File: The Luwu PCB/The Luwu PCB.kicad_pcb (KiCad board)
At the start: 4 copper layers, 38.3 x 104.3 mm, 81 parts, among them IC1 TPS22953DSQR, IC2 ESP32-C3FH4, IC4 CD40109BPWR, IC5 SN74LV1T04DCKRG4, IC6 UCC27519DBVR, IC7 UCC27519DBVR, IC8 UCC27519DBVR, J1 2337019-1, J10 Neopixel Terminal out 3, J2 USB_C_Receptacle_USB2.0, J3 5V_IN, J4 Neopixel Terminal opt 1, J5 12V_IN, J6 V SEL LS, J7 Screw_Terminal_01x04, J8 Neopixel Terminal, J9 Neopixel Terminal opt 2, Q2 BUK7D25-40EX, Q3 BUK7D25-40EX, Q4 BUK7D25-40EX, SW1 PTS636 SP50, SW2 PTS636 SP50, U1 2.4GHZ_PCB_Antenna_AN043, U2 AP2112K-3.3, U3 USBLC6-2SC6, Y1 ECS-400-10-37B2-CKM-TR

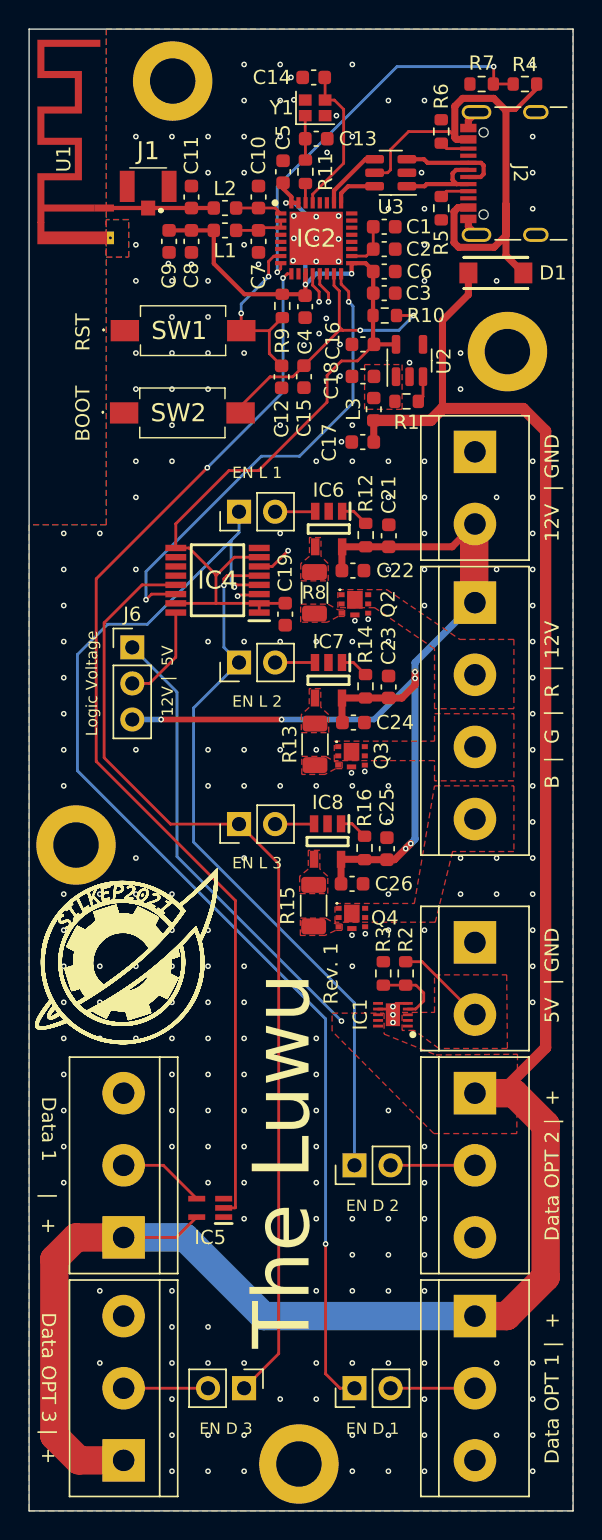
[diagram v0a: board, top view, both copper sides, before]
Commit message: updated size
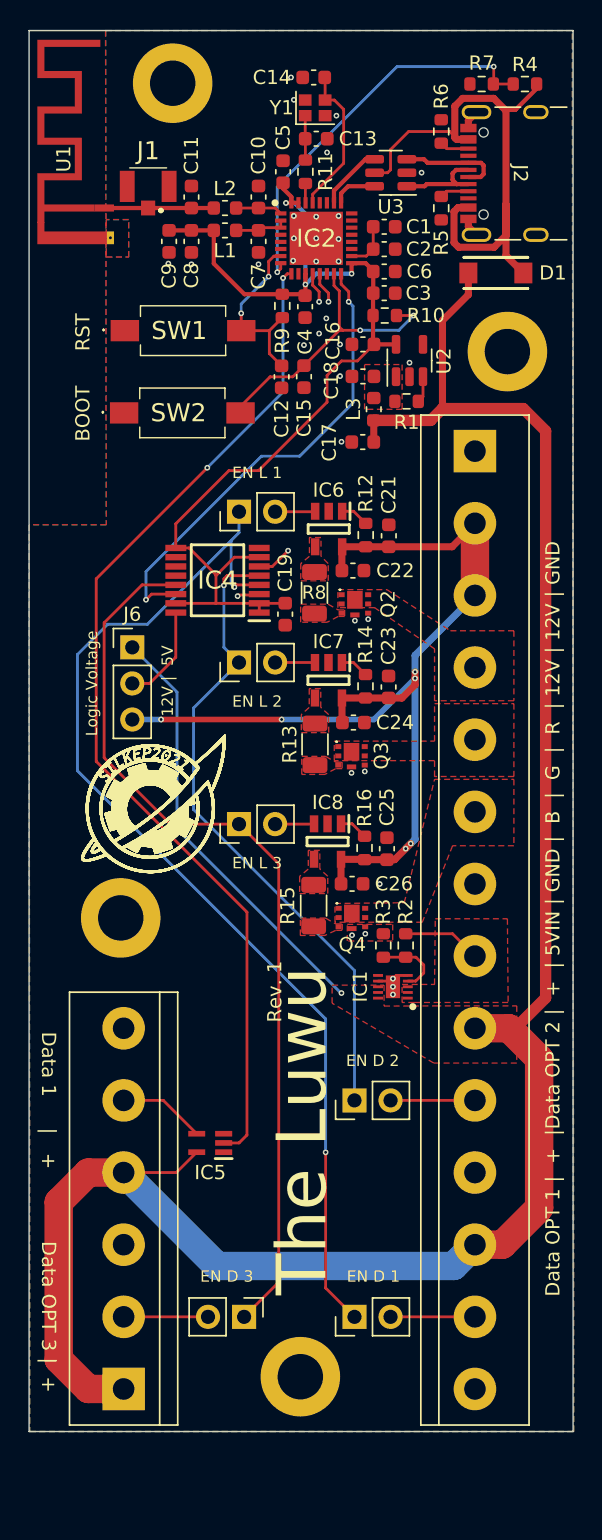
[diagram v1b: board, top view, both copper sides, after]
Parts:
- removed J10: Neopixel Terminal out 3, TerminalBlock:TerminalBlock_bornier-3_P5.08mm
- removed J3: 5V_IN, TerminalBlock:TerminalBlock_bornier-2_P5.08mm
- removed J5: 12V_IN, TerminalBlock:TerminalBlock_bornier-2_P5.08mm
- removed J7: Screw_Terminal_01x04, TerminalBlock:TerminalBlock_bornier-4_P5.08mm
- removed J8: Neopixel Terminal, TerminalBlock:TerminalBlock_bornier-3_P5.08mm
- removed J9: Neopixel Terminal opt 2, TerminalBlock:TerminalBlock_bornier-3_P5.08mm
- added J11: Screw_Terminal_01x14, Connector_custom:TerminalBlock_bornier-14_P5.08mm, F.Cu at (98.2, 111.3)
- J4: value Neopixel Terminal opt 1 -> Screw_Terminal_01x06; footprint TerminalBlock:TerminalBlock_bornier-3_P5.08mm -> TerminalBlock:TerminalBlock_bornier-6_P5.08mm
- moved J4 25.3 mm to (73.5, 146.9), turned to 90 degrees
- moved H3 6.15 mm to (85.9, 146.0)
- moved H1 6.02 mm to (73.3, 113.7)
- moved JP1 5.03 mm to (89.7, 141.8)
- moved JP3 5.03 mm to (81.9, 141.8)
- moved IC5 4.57 mm to (79.6, 129.5)
- moved JP2 4.57 mm to (89.7, 126.5)
- moved IC1 1.97 mm to (92.4, 118.5)
- moved R2 1.97 mm to (93.3, 115.6)
- moved R3 1.97 mm to (91.7, 115.6)
- moved H4 0.15 mm to (76.9, 54.9)
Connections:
- net /5V_IN_TERM renamed 5V_IN_TERM
- IC5 pad 4: /DATA 1 OUT -> DATA 1 OUT
- J4 pad 2: /DATA OPT1 OUT -> DATA OPT3 OUT
- JP1 pad 2: /DATA OPT1 OUT -> DATA OPT1 OUT
- JP2 pad 2: /DATA OPT2 OUT -> DATA OPT2 OUT
- JP3 pad 2: /DATA OPT3 OUT -> DATA OPT3 OUT
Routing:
- net +5V: track 186.1 -> 178.5 mm
- net DATA 1 OUT: track 0.00 -> 6.12 mm
- net /DATA 1 OUT: track 6.12 -> 0.00 mm
- net DATA OPT3 OUT: track 0.00 -> 5.94 mm
- net DATA OPT2 OUT: track 0.00 -> 5.94 mm
- net DATA OPT1 OUT: track 0.00 -> 5.94 mm
- net /DATA OPT3 OUT: track 5.94 -> 0.00 mm
- net /DATA OPT2 OUT: track 5.94 -> 0.00 mm
- net /DATA OPT1 OUT: track 5.94 -> 0.00 mm
- net /DATA OPT1: track 82.0 -> 76.3 mm
- net /DATA OPT3: track 69.0 -> 64.0 mm
- net /DATA OPT2: track 50.3 -> 45.8 mm
- net /DATA 1: track 76.5 -> 72.8 mm
- net 5V_IN_TERM: track 6.42 -> 5.53 mm
- net GND: vias 242 -> 34
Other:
- board size 38.3 x 104.3 mm -> 38.3 x 98.7 mm
- board text added: "Data OPT 1 | + |Data OPT 2 | + | 5VIN | GND | B | G | R | 12V | 12V | GND"
- board text removed: "12V | GND"
- board text removed: "5V | GND"
- board text removed: "B | G | R | 12V"
- board text removed: "Data OPT 1 | +"
- board text removed: "Data OPT 2 | +"
